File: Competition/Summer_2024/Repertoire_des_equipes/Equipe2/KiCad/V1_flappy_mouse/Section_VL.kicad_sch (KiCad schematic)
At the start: 14 parts, among them J301 ESP_GAUCHE, J302 ESP_DROIT, J303 CAPACITIVE, J304 Conn_01x08_Pin, U301 LM393

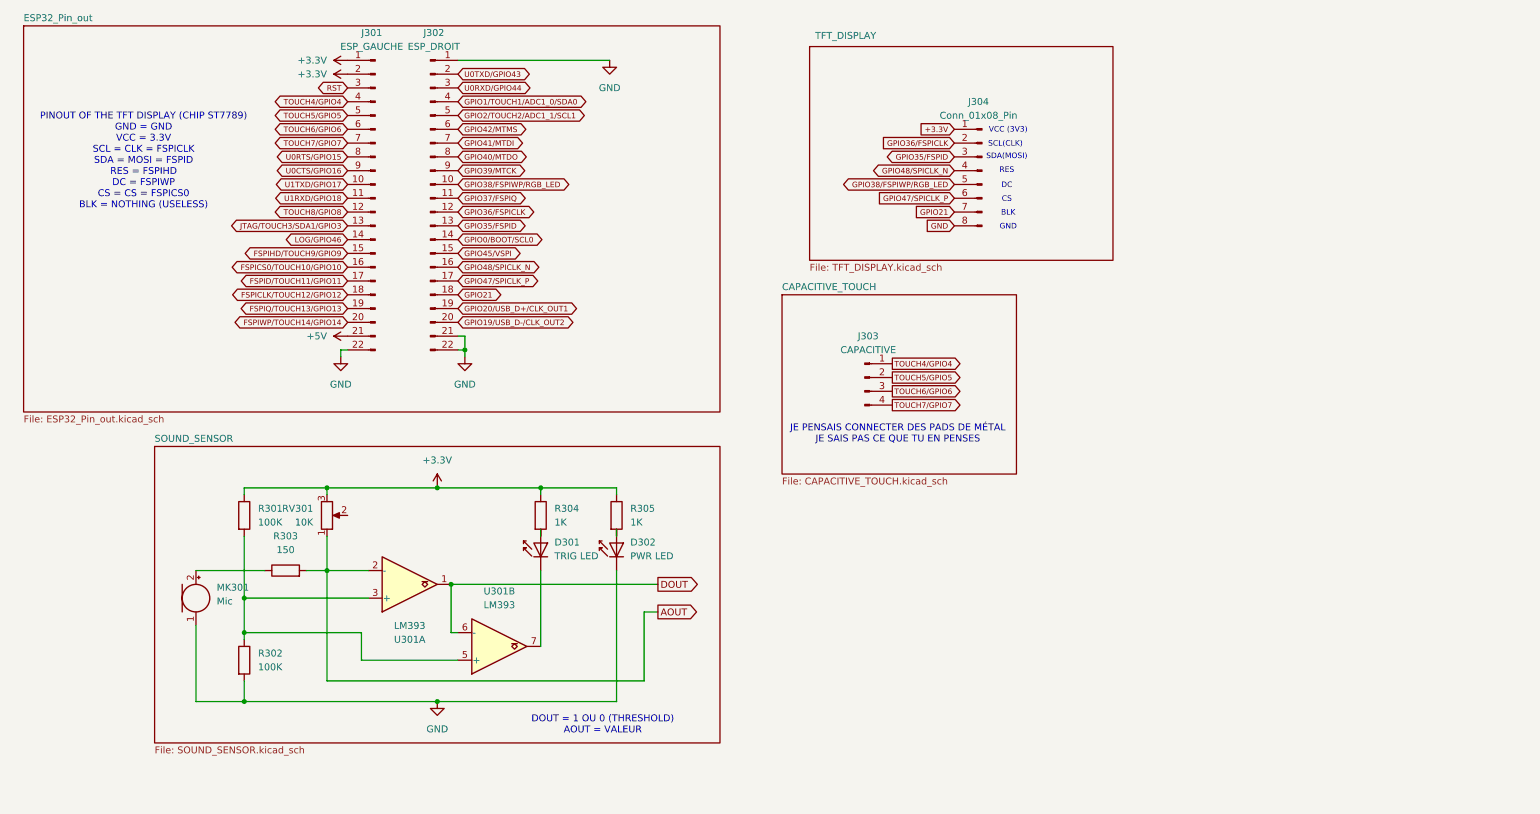
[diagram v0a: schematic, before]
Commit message: Taking a break, i will come back later today
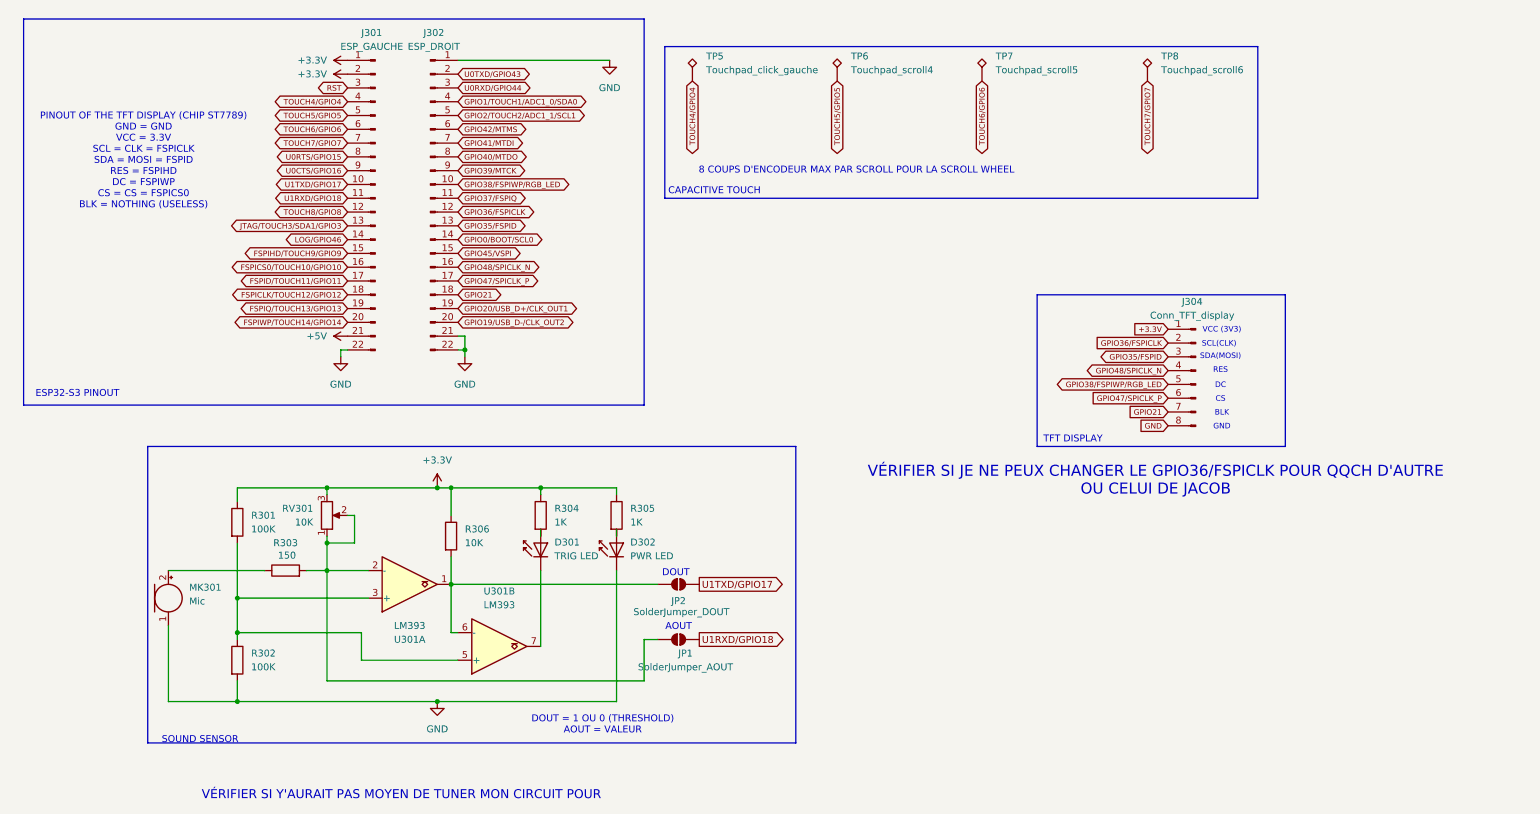
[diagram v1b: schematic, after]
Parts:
- removed J303: CAPACITIVE, symbol Connector:Conn_01x04_Pin
- added JP1: SolderJumper_AOUT, symbol Jumper:SolderJumper_2_Open
- added JP2: SolderJumper_DOUT, symbol Jumper:SolderJumper_2_Open
- added R306: 10K, symbol Device:R
- added TP5: Touchpad_click_gauche, Librairie_touchpad:Touchpad_biz_rect, symbol Connector:TestPoint_Alt
- added TP6: Touchpad_scroll4, Librairie_touchpad:Touchpad_biz_rect, symbol Connector:TestPoint_Alt
- added TP7: Touchpad_scroll5, Librairie_touchpad:Touchpad_biz_rect, symbol Connector:TestPoint_Alt
- added TP8: Touchpad_scroll6, Librairie_touchpad:Touchpad_biz_rect, symbol Connector:TestPoint_Alt
- J304: value Conn_01x08_Pin -> Conn_TFT_display
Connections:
- net AOUT is gone; now on an unnamed net: R303.2, RV301.1, U301.2 (-)
- net +3.3V: now also R306.1
- net TOUCH4/GPIO4: now also TP5.1
- net TOUCH5/GPIO5: now also TP6.1
- net TOUCH6/GPIO6: now also TP7.1
- net TOUCH7/GPIO7: now also TP8.1
- net U1RXD/GPIO18: now also JP1.2 (B)
- net U1TXD/GPIO17: now also JP2.2 (B)
- net at RV301.2: now also JP1.1 (A)
- net DOUT: no longer names the net of U301.1, U301.6 (-)
- net DOUT: now also JP2.1 (A), R306.2
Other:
- removed sheet CAPACITIVE_TOUCH
- removed sheet ESP32_Pin_out
- removed sheet SOUND_SENSOR
- removed sheet TFT_DISPLAY
- note added: "8 COUPS D'ENCODEUR MAX PAR SCROLL POUR LA SCROLL WHEEL"
- note added: "AOUT"
- note added: "CAPACITIVE TOUCH"
- note added: "DOUT"
- note added: "ESP32-S3 PINOUT"
- note added: "SOUND SENSOR"
- note added: "TFT DISPLAY"
- note added: "VÉRIFIER SI JE NE PEUX CHANGER LE GPIO36/FSPICLK POUR QQCH D'AUTRE OU CELUI DE JACOB"
- note added: "VÉRIFIER SI Y'AURAIT PAS MOYEN DE TUNER MON CIRCUIT POUR"
- note removed: "JE PENSAIS CONNECTER DES PADS DE MÉTAL JE SAIS PAS CE QUE TU EN PENSES"
- moved on the sheet: J304, MK301, R301, R302
